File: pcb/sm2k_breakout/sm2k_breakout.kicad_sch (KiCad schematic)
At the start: 3 parts

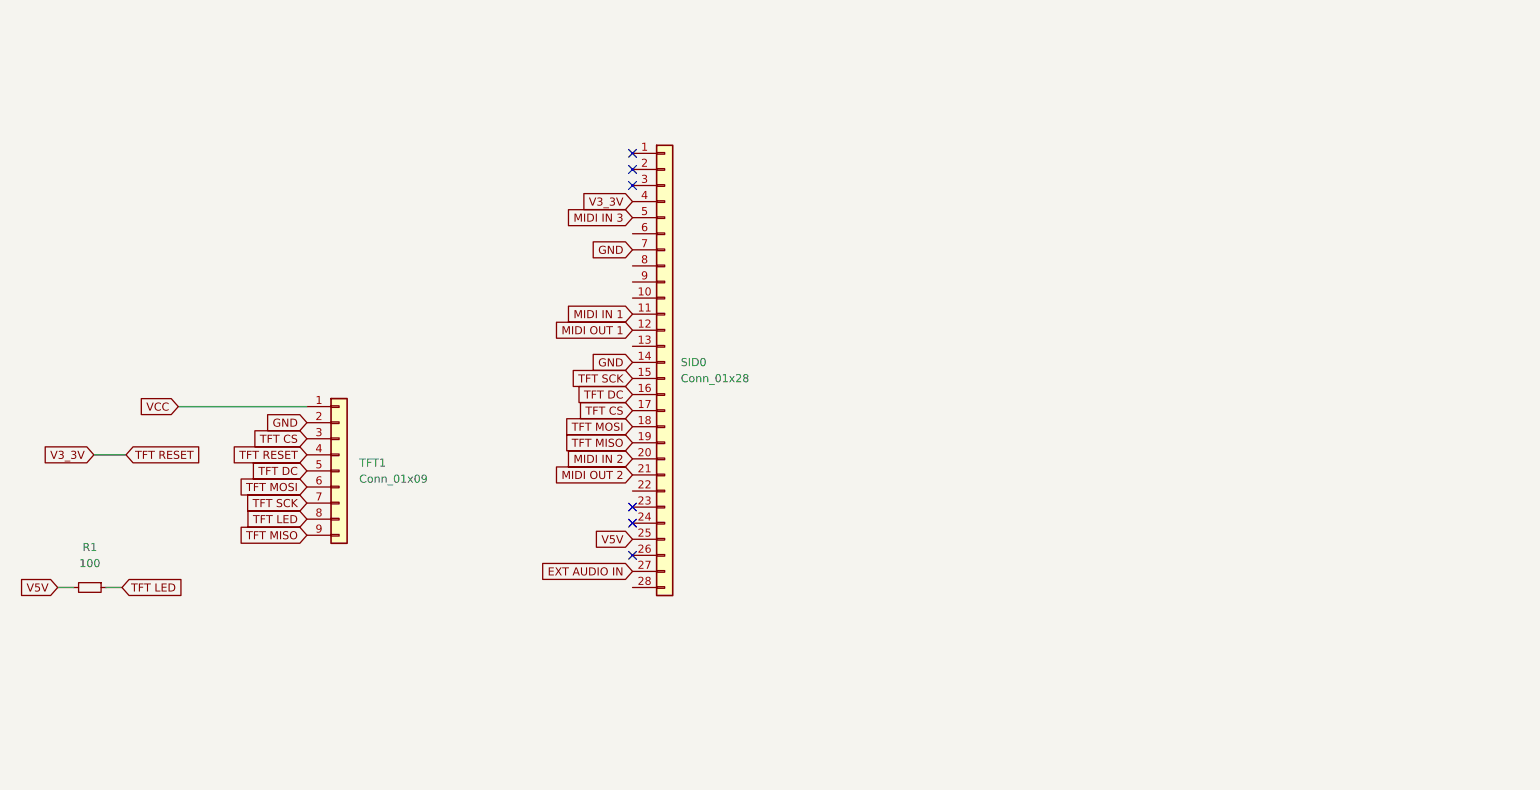
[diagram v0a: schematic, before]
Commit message: button matrix
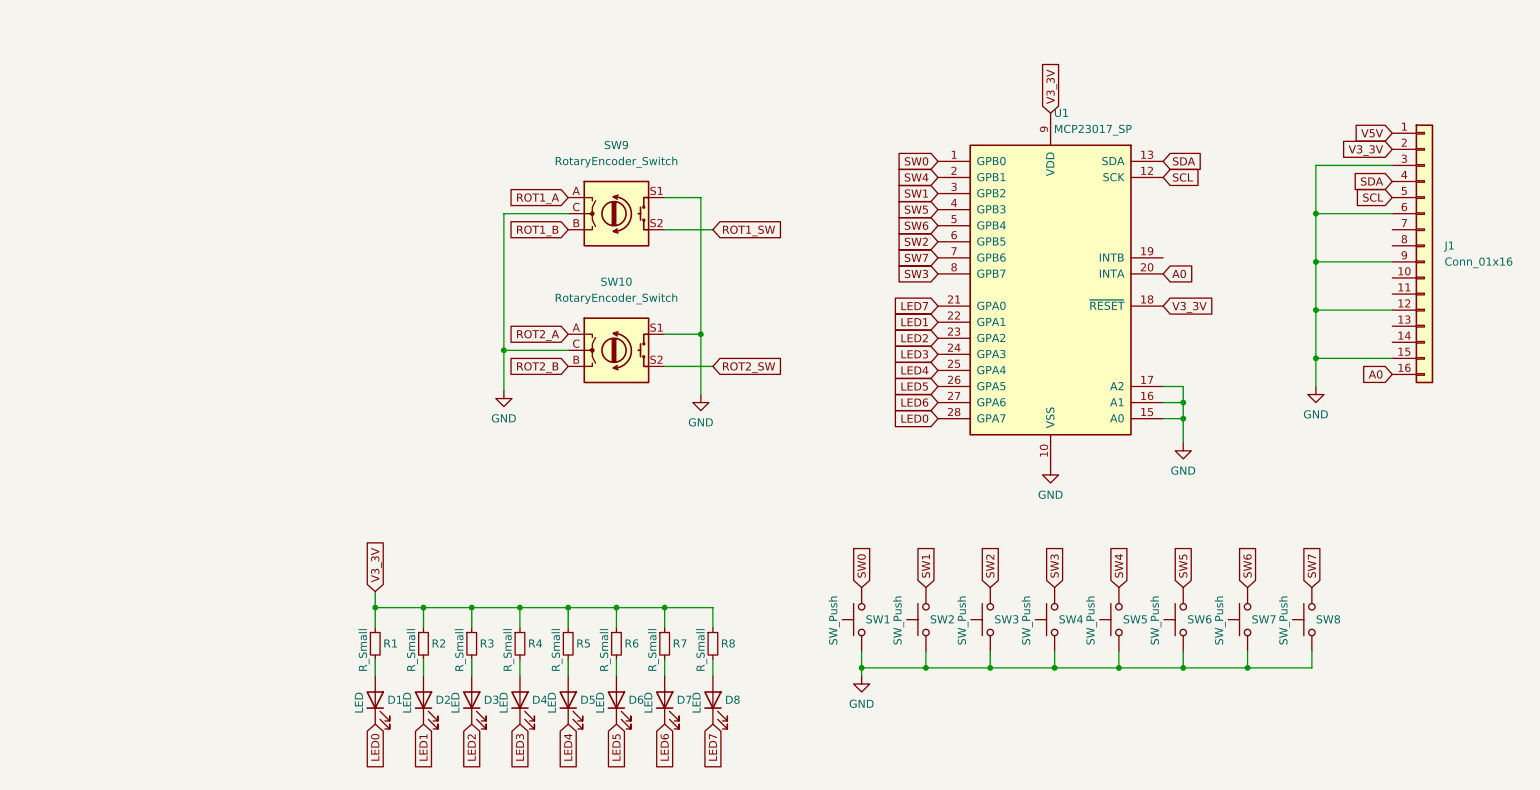
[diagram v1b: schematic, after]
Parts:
- removed SID0: Conn_01x28, Package_DIP:DIP-28_W15.24mm_Socket, symbol Connector_Generic:Conn_01x28
- removed TFT1: Conn_01x09, Connector_PinHeader_2.54mm:PinHeader_1x09_P2.54mm_Vertical, symbol Connector_Generic:Conn_01x09
- added D1, D2, D3, D4, D5, D6, D7, D8: LED, LED_THT:LED_D3.0mm, symbol Device:LED
- added J1: Conn_01x16, Connector_IDC:IDC-Header_2x08_P2.54mm_Vertical, symbol Connector_Generic:Conn_01x16
- added R2, R3, R4, R5, R6, R7, R8: R_Small, Resistor_SMD:R_0603_1608Metric_Pad0.98x0.95mm_HandSolder, symbol Device:R_Small
- added SW1, SW2, SW3, SW4, SW5, SW6, SW7, SW8: SW_Push, Button_Switch_Keyboard:SW_Cherry_MX_1.00u_PCB, symbol Switch:SW_Push
- added SW10, SW9: RotaryEncoder_Switch, Rotary_Encoder:RotaryEncoder_Alps_EC11E-Switch_Vertical_H20mm_CircularMountingHoles, symbol Device:RotaryEncoder_Switch
- added U1: MCP23017_SP, Package_DIP:DIP-28_W7.62mm, symbol Interface_Expansion:MCP23017_SP
- R1: value 100 -> R_Small
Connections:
- net GND: now also J1.12 (Pin_12), J1.15 (Pin_15), J1.3 (Pin_3), J1.6 (Pin_6), J1.9 (Pin_9), SW1.1, SW10.C, SW10.S1, SW2.1, SW3.1, SW4.1, SW5.1, SW6.1, SW7.1, SW8.1, SW9.C, SW9.S1, U1.10 (VSS), U1.15 (A0), U1.16 (A1), U1.17 (A2)
- net V5V: now also J1.1 (Pin_1); no longer R1.2
- net TFT LED renamed V3_3V
- net V3_3V: now also J1.2 (Pin_2), R2.1, R3.1, R4.1, R5.1, R6.1, R7.1, R8.1, U1.18 (~{RESET}), U1.9 (VDD)
- new net: D2.2 (A), R2.2
- new net: D5.2 (A), R5.2
- new net: D1.2 (A), R1.2
- new net: D8.2 (A), R8.2
- new net: D3.2 (A), R3.2
- new net: D6.2 (A), R6.2
- new net: D7.2 (A), R7.2
- new net: D4.2 (A), R4.2
- new net A0: J1.16 (Pin_16), U1.20 (INTA)
- new net LED0: D1.1 (K), U1.28 (GPA7)
- new net LED1: D2.1 (K), U1.22 (GPA1)
- new net LED2: D3.1 (K), U1.23 (GPA2)
- new net LED3: D4.1 (K), U1.24 (GPA3)
- new net LED4: D5.1 (K), U1.25 (GPA4)
- new net LED5: D6.1 (K), U1.26 (GPA5)
- new net LED6: D7.1 (K), U1.27 (GPA6)
- new net LED7: D8.1 (K), U1.21 (GPA0)
- new net ROT1_A: SW9.A
- new net ROT1_B: SW9.B
- new net ROT1_SW: SW9.S2
- new net ROT2_A: SW10.A
- new net ROT2_B: SW10.B
- new net ROT2_SW: SW10.S2
- new net SCL: J1.5 (Pin_5), U1.12 (SCK)
- new net SDA: J1.4 (Pin_4), U1.13 (SDA)
- new net SW0: SW1.2, U1.1 (GPB0)
- new net SW1: SW2.2, U1.3 (GPB2)
- new net SW2: SW3.2, U1.6 (GPB5)
- new net SW3: SW4.2, U1.8 (GPB7)
- new net SW4: SW5.2, U1.2 (GPB1)
- new net SW5: SW6.2, U1.4 (GPB3)
- new net SW6: SW7.2, U1.5 (GPB4)
- new net SW7: SW8.2, U1.7 (GPB6)
- no-connect marks 6 -> 0

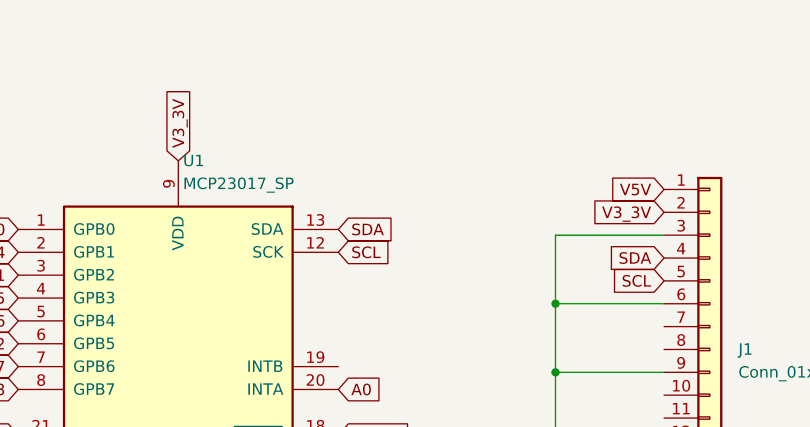
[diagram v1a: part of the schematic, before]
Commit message: Ui fixes
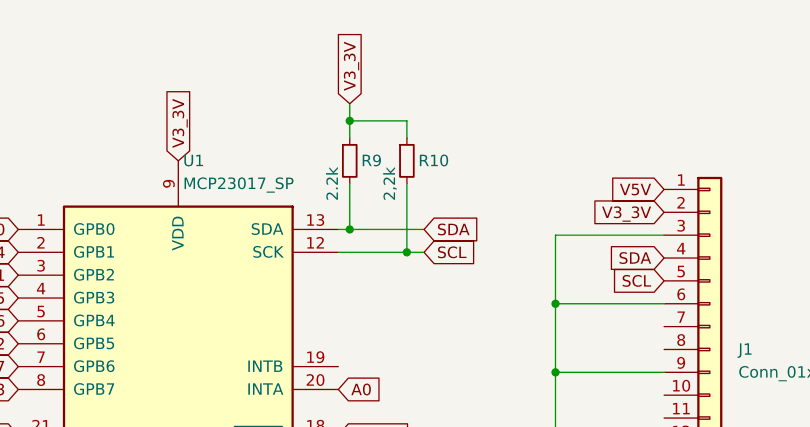
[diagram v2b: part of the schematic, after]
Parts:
- added R10: 2,2k, Resistor_SMD:R_0603_1608Metric_Pad0.98x0.95mm_HandSolder, symbol Device:R_Small
- added R9: 2.2k, Resistor_SMD:R_0603_1608Metric_Pad0.98x0.95mm_HandSolder, symbol Device:R_Small
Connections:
- net SCL: now also R10.2
- net SDA: now also R9.2
- net V3_3V: now also R10.1, R9.1
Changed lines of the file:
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@@
   (junction (at 111.76 121.285) (diameter 0) (color 0 0 0 0)
   )
+  (junction (at 220.98 53.34) (diameter 0) (color 0 0 0 0)
+  )
   (junction (at 134.62 121.285) (diameter 0) (color 0 0 0 0)
   )
@@
   (junction (at 196.215 130.81) (diameter 0) (color 0 0 0 0)
   )
+  (junction (at 214.63 38.735) (diameter 0) (color 0 0 0 0)
+  )
   (junction (at 109.22 80.645) (diameter 0) (color 0 0 0 0)
   )
@@
   (junction (at 206.375 130.81) (diameter 0) (color 0 0 0 0)
   )
+  (junction (at 214.63 50.8) (diameter 0) (color 0 0 0 0)
+  )
   (wire (pts (xy 104.14 121.285) (xy 96.52 121.285))
     (stroke (width 0) (type default) (color 0 0 0 0))
@@
     (stroke (width 0) (type default) (color 0 0 0 0))
   )
+  (wire (pts (xy 220.98 53.34) (xy 222.885 53.34))
+    (stroke (width 0) (type default) (color 0 0 0 0))
+  )
   (wire (pts (xy 109.22 86.995) (xy 109.22 80.645))
     (stroke (width 0) (type default) (color 0 0 0 0))
@@
     (stroke (width 0) (type default) (color 0 0 0 0))
   )
+  (wire (pts (xy 214.63 45.72) (xy 214.63 50.8))
+    (stroke (width 0) (type default) (color 0 0 0 0))
+  )
   (wire (pts (xy 213.36 86.36) (xy 216.535 86.36))
     (stroke (width 0) (type default) (color 0 0 0 0))
@@
     (stroke (width 0) (type default) (color 0 0 0 0))
   )
+  (wire (pts (xy 214.63 38.735) (xy 220.98 38.735))
+    (stroke (width 0) (type default) (color 0 0 0 0))
+  )
   (wire (pts (xy 237.49 66.675) (xy 237.49 74.295))
     (stroke (width 0) (type default) (color 0 0 0 0))
   )
+  (wire (pts (xy 214.63 36.83) (xy 214.63 38.735))
+    (stroke (width 0) (type default) (color 0 0 0 0))
+  )
   (wire (pts (xy 104.14 129.54) (xy 104.14 132.08))
     (stroke (width 0) (type default) (color 0 0 0 0))
@@
     (stroke (width 0) (type default) (color 0 0 0 0))
   )
+  (wire (pts (xy 213.36 50.8) (xy 214.63 50.8))
+    (stroke (width 0) (type default) (color 0 0 0 0))
+  )
   (wire (pts (xy 237.49 59.055) (xy 237.49 66.675))
     (stroke (width 0) (type default) (color 0 0 0 0))
@@
     (stroke (width 0) (type default) (color 0 0 0 0))
   )
+  (wire (pts (xy 214.63 38.735) (xy 214.63 40.64))
+    (stroke (width 0) (type default) (color 0 0 0 0))
+  )
   (wire (pts (xy 119.38 129.54) (xy 119.38 132.08))
     (stroke (width 0) (type default) (color 0 0 0 0))
@@
     (stroke (width 0) (type default) (color 0 0 0 0))
   )
+  (wire (pts (xy 213.36 53.34) (xy 220.98 53.34))
+    (stroke (width 0) (type default) (color 0 0 0 0))
+  )
   (wire (pts (xy 249.555 59.055) (xy 237.49 59.055))
     (stroke (width 0) (type default) (color 0 0 0 0))
@@
     (stroke (width 0) (type default) (color 0 0 0 0))
   )
+  (wire (pts (xy 220.98 38.735) (xy 220.98 40.64))
+    (stroke (width 0) (type default) (color 0 0 0 0))
+  )
   (wire (pts (xy 109.22 80.645) (xy 109.22 59.055))
     (stroke (width 0) (type default) (color 0 0 0 0))
@@
     (stroke (width 0) (type default) (color 0 0 0 0))
   )
+  (wire (pts (xy 220.98 45.72) (xy 220.98 53.34))
+    (stroke (width 0) (type default) (color 0 0 0 0))
+  )
   (wire (pts (xy 237.49 74.295) (xy 237.49 81.915))
+    (stroke (width 0) (type default) (color 0 0 0 0))
+  )
+  (wire (pts (xy 214.63 50.8) (xy 222.885 50.8))
     (stroke (width 0) (type default) (color 0 0 0 0))
   )
@@
     )
   )
-  (global_label "SCL" (shape input) (at 213.36 53.34 0) (fields_autoplaced)
-    (effects (font (size 1.27 1.27)) (justify left))
-    (property "Intersheet References" "${INTERSHEET_REFS}" (id 0) (at 219.2807 53.4194 0)
+  (global_label "SCL" (shape input) (at 222.885 53.34 0) (fields_autoplaced)
+    (effects (font (size 1.27 1.27)) (justify left))
+    (property "Intersheet References" "${INTERSHEET_REFS}" (id 0) (at 228.8057 53.4194 0)
       (effects (font (size 1.27 1.27)) (justify left) hide)
     )
@@
     )
   )
-  (global_label "SDA" (shape input) (at 213.36 50.8 0) (fields_autoplaced)
-    (effects (font (size 1.27 1.27)) (justify left))
-    (property "Intersheet References" "${INTERSHEET_REFS}" (id 0) (at 219.3412 50.8794 0)
+  (global_label "SDA" (shape input) (at 222.885 50.8 0) (fields_autoplaced)
+    (effects (font (size 1.27 1.27)) (justify left))
+    (property "Intersheet References" "${INTERSHEET_REFS}" (id 0) (at 228.8662 50.8794 0)
       (effects (font (size 1.27 1.27)) (justify left) hide)
     )
@@
     )
   )
+  (global_label "V3_3V" (shape input) (at 214.63 36.83 90) (fields_autoplaced)
+    (effects (font (size 1.27 1.27)) (justify left))
+    (property "Intersheet References" "${INTERSHEET_REFS}" (id 0) (at 214.7094 28.8531 90)
+      (effects (font (size 1.27 1.27)) (justify left) hide)
+    )
+  )
   (symbol (lib_id "Device:LED") (at 96.52 135.89 90) (unit 1)
     (in_bom yes) (on_board yes)
@@
     )
     (property "Datasheet" "~" (id 3) (at 119.38 127 0)
+      (effects (font (size 1.27 1.27)) hide)
+    )
+    (pin "1")
+    (pin "2")
+  )
+  (symbol (lib_id "Device:R_Small") (at 220.98 43.18 0) (unit 1)
+    (in_bom yes) (on_board yes)
+    (property "Reference" "R10" (id 0) (at 222.25 43.18 0)
+      (effects (font (size 1.27 1.27)) (justify left))
+    )
+    (property "Value" "2,2k" (id 1) (at 219.075 47.625 90)
+      (effects (font (size 1.27 1.27)) (justify left))
+    )
+    (property "Footprint" "Resistor_SMD:R_0603_1608Metric_Pad0.98x0.95mm_HandSolder" (id 2) (at 220.98 43.18 0)
+      (effects (font (size 1.27 1.27)) hide)
+    )
+    (property "Datasheet" "~" (id 3) (at 220.98 43.18 0)
       (effects (font (size 1.27 1.27)) hide)
     )
@@
     )
     (property "Datasheet" "~" (id 3) (at 88.9 127 0)
+      (effects (font (size 1.27 1.27)) hide)
+    )
+    (pin "1")
+    (pin "2")
+  )
+  (symbol (lib_id "Device:R_Small") (at 214.63 43.18 0) (unit 1)
+    (in_bom yes) (on_board yes)
+    (property "Reference" "R9" (id 0) (at 215.9 43.18 0)
+      (effects (font (size 1.27 1.27)) (justify left))
+    )
+    (property "Value" "2.2k" (id 1) (at 212.725 47.625 90)
+      (effects (font (size 1.27 1.27)) (justify left))
+    )
+    (property "Footprint" "Resistor_SMD:R_0603_1608Metric_Pad0.98x0.95mm_HandSolder" (id 2) (at 214.63 43.18 0)
+      (effects (font (size 1.27 1.27)) hide)
+    )
+    (property "Datasheet" "~" (id 3) (at 214.63 43.18 0)
       (effects (font (size 1.27 1.27)) hide)
     )
@@
       (reference "R8") (unit 1) (value "R_Small") (footprint "Resistor_SMD:R_0603_1608Metric_Pad0.98x0.95mm_HandSolder")
     )
+    (path "/3900a3b0-431b-4976-9497-7ceb8bad1232"
+      (reference "R9") (unit 1) (value "2.2k") (footprint "Resistor_SMD:R_0603_1608Metric_Pad0.98x0.95mm_HandSolder")
+    )
+    (path "/0985b497-b03a-4484-9da9-bc0206e0cfbd"
+      (reference "R10") (unit 1) (value "2,2k") (footprint "Resistor_SMD:R_0603_1608Metric_Pad0.98x0.95mm_HandSolder")
+    )
     (path "/88e3af35-e975-415d-96f3-bb80150de8bc"
